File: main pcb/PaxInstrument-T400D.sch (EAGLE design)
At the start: 88 parts, among them IC2 NC7S00DBV, J1 MICRO-SDCARD-CONNECTOR-330006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, Q1 DMP2035U-7, U2 APX809, U3 MCP73831, U4 MIC5219-3.3V, X1 FH12-12S-1S, X2 FH12-12S-0.5SH, Y1 RESONATORSMD

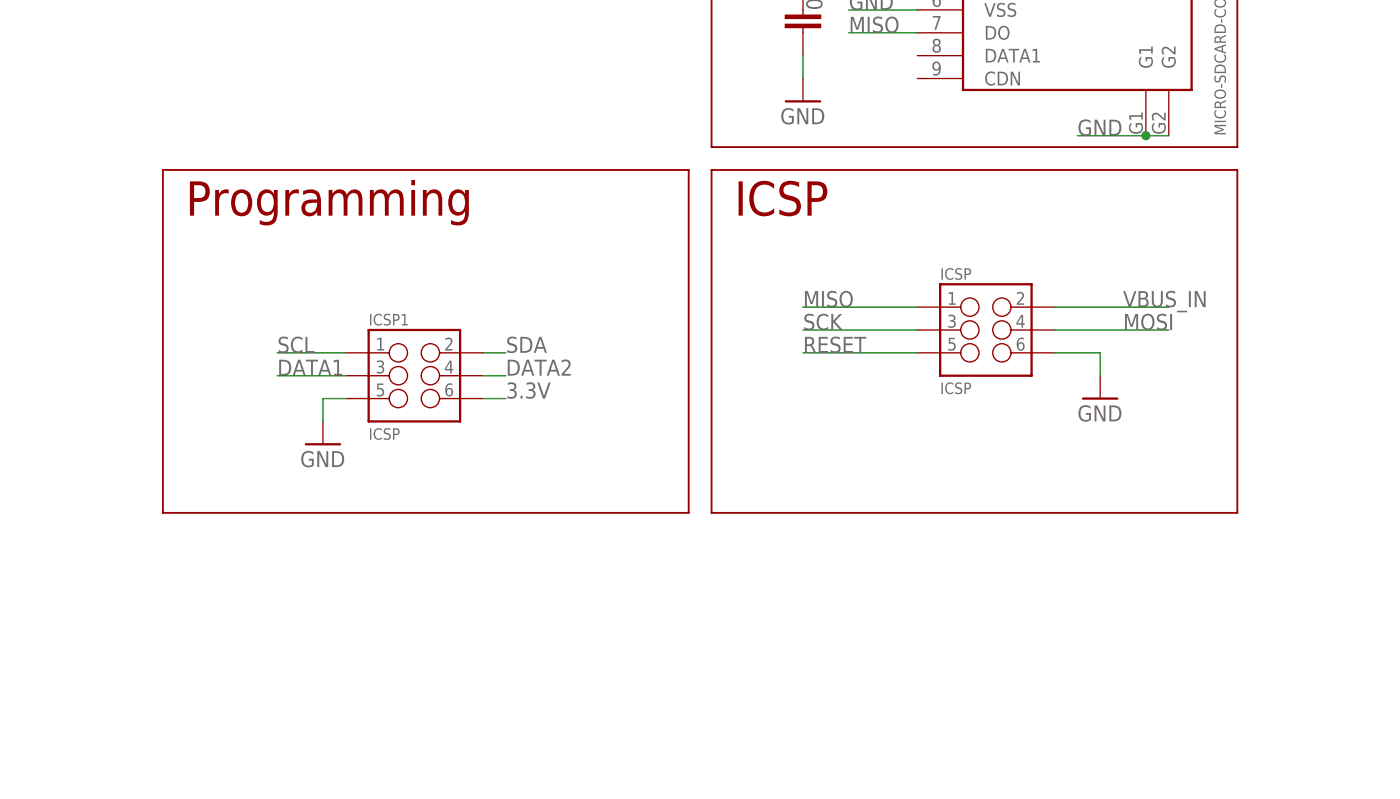
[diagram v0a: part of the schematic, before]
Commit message: - Not sure what changed. This is still just playing around.
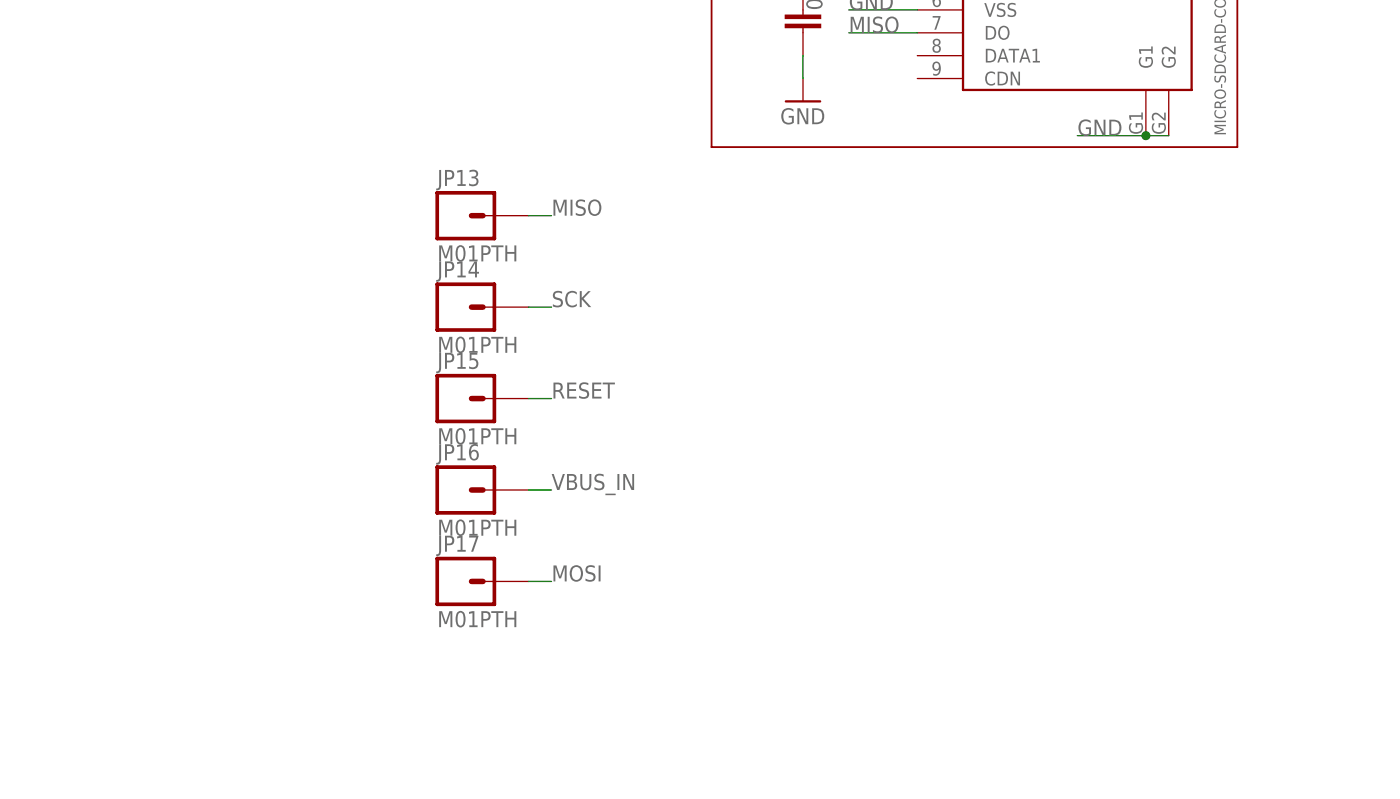
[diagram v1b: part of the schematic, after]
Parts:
- removed ICSP, ICSP1: ICSP, PaxInstrument-T400:SPARKFUN-CONNECTORS_M03X2PAX
- added JP13, JP14, JP15, JP16, JP17: M01PTH, SparkFun-Connectors:M01PTH
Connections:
- net 3.3V: no longer ICSP1.6
- net DATA1: no longer ICSP1.3
- net DATA2: no longer ICSP1.4
- net GND: no longer ICSP.6, ICSP1.5
- net MISO: now also JP13.1; no longer ICSP.1
- net MOSI: now also JP17.1; no longer ICSP.4
- net RESET: now also JP15.1; no longer ICSP.5
- net SCK: now also JP14.1; no longer ICSP.3
- net SCL: no longer ICSP1.1
- net SDA: no longer ICSP1.2
- net VBUS_IN: now also JP16.1; no longer ICSP.2
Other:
- note removed: "ICSP"
- note removed: "Programming"
